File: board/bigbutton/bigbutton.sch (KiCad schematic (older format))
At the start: 55 parts, among them J1 SWD, J2 USB_C_Receptacle_USB2.0, SW1 RESET, SW2 SMOL, SW3 LORGE, U1 STM32F302CBTx, U2 ATECC608A-SSHDA, U3 WE-TVS-82400102, X1 16MHz

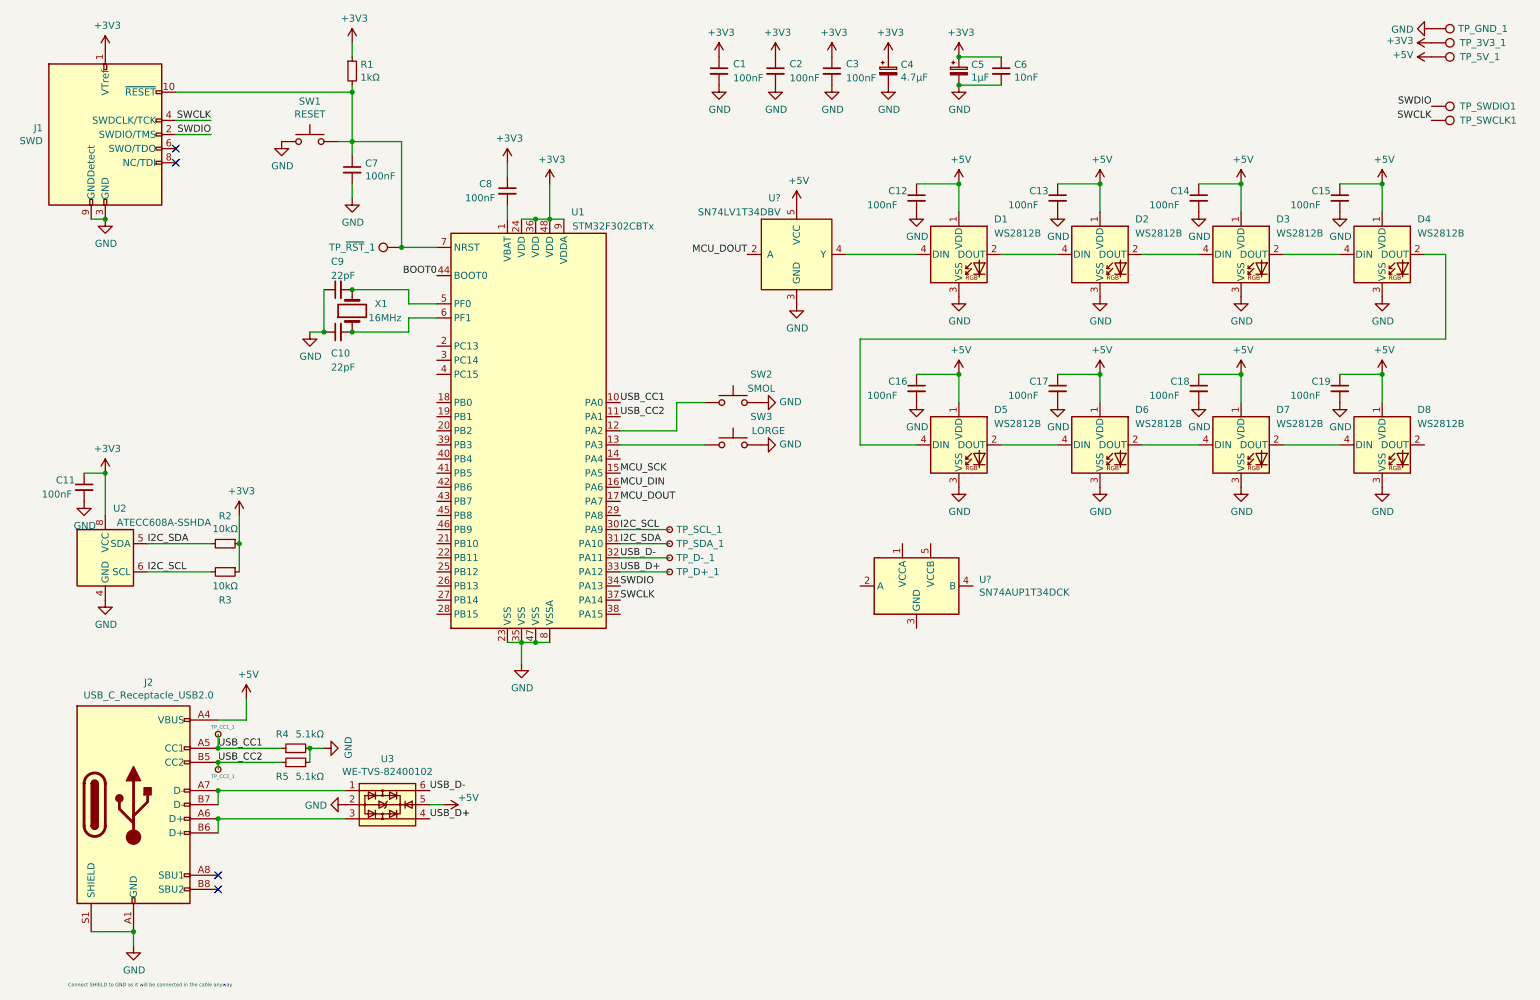
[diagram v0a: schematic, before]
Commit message: Add vreg
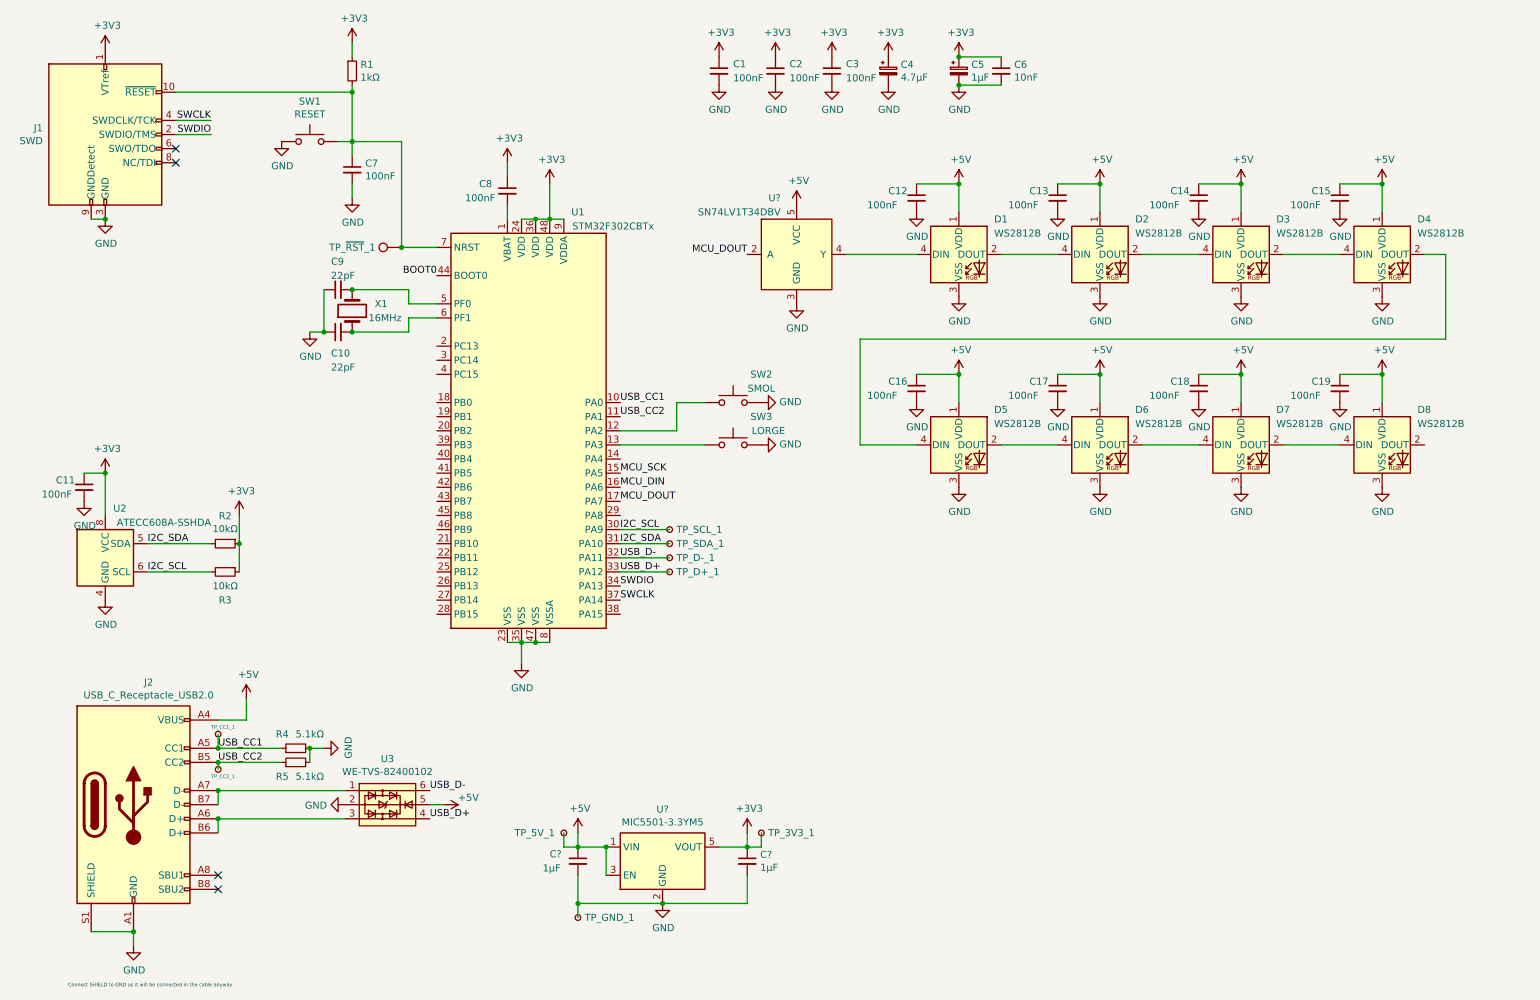
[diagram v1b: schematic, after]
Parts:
- removed TP_3V3_1, TP_5V_1, TP_GND_1, TP_SWCLK1, TP_SWDIO1: TestPoint, symbol Connector:TestPoint
- removed U?: SN74AUP1T34DCK, Package_TO_SOT_SMD:SOT-353_SC-70-5, symbol Logic_LevelTranslator:SN74AUP1T34DCK
- added C? (x2): 1µF, symbol Device:C_Small
- added TP_3V3_1, TP_5V_1, TP_GND_1: TestPoint_Small, symbol Connector:TestPoint_Small
- added U?: MIC5501-3.3YM5, Package_TO_SOT_SMD:SOT-23-5, symbol Regulator_Linear:MIC5501-3.0YM5
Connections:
- net +3V3: now also C?.1, TP_3V3_1.1, U?.5 (VOUT)
- net +5V: now also C?.1, TP_5V_1.1, U?.1 (VIN), U?.3 (EN)
- net GND: now also C?.2, C?.2, TP_GND_1.1, U?.2 (GND)
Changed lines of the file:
@@
 Text Label 4800 4150 0    50   ~ 0
 I2C_SCL
-$Comp
-L Connector:TestPoint TP_SWDIO1
-U 1 1 5F610285
-P 10550 1150
-F 0 "TP_SWDIO1" V 10550 1350 50  0000 L CNN
-F 1 "TestPoint" V 10595 1338 50  0001 L CNN
-F 2 "" H 10750 1150 50  0001 C CNN
-F 3 "~" H 10750 1150 50  0001 C CNN
-	1    10550 1150
-	0    1    1    0
-$EndComp
-$Comp
-L Connector:TestPoint TP_SWCLK1
-U 1 1 5F610307
-P 10550 1250
-F 0 "TP_SWCLK1" V 10550 1450 50  0000 L CNN
-F 1 "TestPoint" V 10595 1438 50  0001 L CNN
-F 2 "" H 10750 1250 50  0001 C CNN
-F 3 "~" H 10750 1250 50  0001 C CNN
-	1    10550 1250
-	0    1    1    0
-$EndComp
-Text Label 10550 1150 2    50   ~ 0
-SWDIO
-Text Label 10550 1250 2    50   ~ 0
-SWCLK
 Text Label 4800 4350 0    50   ~ 0
 USB_D-
@@
 Text Label 4800 3750 0    50   ~ 0
 MCU_SCK
-$Comp
-L Connector:TestPoint TP_GND_1
-U 1 1 5F63CA5F
-P 10550 600
-F 0 "TP_GND_1" V 10550 788 50  0000 L CNN
-F 1 "TestPoint" V 10595 788 50  0001 L CNN
-F 2 "" H 10750 600 50  0001 C CNN
-F 3 "~" H 10750 600 50  0001 C CNN
-	1    10550 600
-	0    1    1    0
-$EndComp
-$Comp
-L power:GND #PWR01
-U 1 1 5F63D061
-P 10550 600
-F 0 "#PWR01" H 10550 350 50  0001 C CNN
-F 1 "GND" V 10555 472 50  0000 R CNN
-F 2 "" H 10550 600 50  0001 C CNN
-F 3 "" H 10550 600 50  0001 C CNN
-	1    10550 600
-	0    1    1    0
-$EndComp
-$Comp
-L Connector:TestPoint TP_3V3_1
-U 1 1 5F63F10F
-P 10550 700
-F 0 "TP_3V3_1" V 10550 900 50  0000 L CNN
-F 1 "TestPoint" V 10595 888 50  0001 L CNN
-F 2 "" H 10750 700 50  0001 C CNN
-F 3 "~" H 10750 700 50  0001 C CNN
-	1    10550 700
-	0    1    1    0
-$EndComp
-$Comp
-L power:+3V3 #PWR03
-U 1 1 5F63F709
-P 10550 700
-F 0 "#PWR03" H 10550 550 50  0001 C CNN
-F 1 "+3V3" V 10565 828 50  0000 L CNN
-F 2 "" H 10550 700 50  0001 C CNN
-F 3 "" H 10550 700 50  0001 C CNN
-	1    10550 700
-	0    -1   -1   0
-$EndComp
-$Comp
-L Connector:TestPoint TP_5V_1
-U 1 1 5F63F82F
-P 10550 800
-F 0 "TP_5V_1" V 10550 1000 50  0000 L CNN
-F 1 "TestPoint" V 10595 988 50  0001 L CNN
-F 2 "" H 10750 800 50  0001 C CNN
-F 3 "~" H 10750 800 50  0001 C CNN
-	1    10550 800
-	0    1    1    0
-$EndComp
-$Comp
-L power:+5V #PWR09
-U 1 1 5F63FFC3
-P 10550 800
-F 0 "#PWR09" H 10550 650 50  0001 C CNN
-F 1 "+5V" V 10565 928 50  0000 L CNN
-F 2 "" H 10550 800 50  0001 C CNN
-F 3 "" H 10550 800 50  0001 C CNN
-	1    10550 800
-	0    -1   -1   0
-$EndComp
 Wire Wire Line
 	4100 1950 4200 1950
@@
 	6400 2200 6900 2200
 $Comp
-L Logic_LevelTranslator:SN74AUP1T34DCK U?
-U 1 1 5F79F9D3
-P 6900 4550
-F 0 "U?" H 7344 4596 50  0000 L CNN
-F 1 "SN74AUP1T34DCK" H 7344 4505 50  0000 L CNN
-F 2 "Package_TO_SOT_SMD:SOT-353_SC-70-5" H 6900 3850 50  0001 C CNN
-F 3 "http://www.ti.com/lit/ds/symlink/sn74aup1t34.pdf" H 6900 3950 50  0001 C CNN
-	1    6900 4550
-	1    0    0    -1
-$EndComp
-$Comp
 L bigbutton:SN74LV1T34DBV U?
 U 1 1 5F7A4DA0
@@
 	1    0    0    -1
 $EndComp
+$Comp
+L Regulator_Linear:MIC5501-3.0YM5 U?
+U 1 1 5F7ACD40
+P 5100 6500
+F 0 "U?" H 5100 6867 50  0000 C CNN
+F 1 "MIC5501-3.3YM5" H 5100 6776 50  0000 C CNN
+F 2 "Package_TO_SOT_SMD:SOT-23-5" H 5100 6100 50  0001 C CNN
+F 3 "http://ww1.microchip.com/downloads/en/DeviceDoc/MIC550X.pdf" H 4850 6750 50  0001 C CNN
+	1    5100 6500
+	1    0    0    -1
+$EndComp
+Wire Wire Line
+	4700 6400 4700 6600
+Wire Wire Line
+	4700 6400 4500 6400
+Wire Wire Line
+	4500 6400 4500 6300
+Connection ~ 4700 6400
+$Comp
+L power:+5V #PWR?
+U 1 1 5F7B4962
+P 4500 6300
+F 0 "#PWR?" H 4500 6150 50  0001 C CNN
+F 1 "+5V" H 4515 6473 50  0000 C CNN
+F 2 "" H 4500 6300 50  0001 C CNN
+F 3 "" H 4500 6300 50  0001 C CNN
+	1    4500 6300
+	1    0    0    -1
+$EndComp
+Wire Wire Line
+	5500 6400 5700 6400
+Wire Wire Line
+	5700 6400 5700 6300
+$Comp
+L power:+3V3 #PWR?
+U 1 1 5F7B7EC3
+P 5700 6300
+F 0 "#PWR?" H 5700 6150 50  0001 C CNN
+F 1 "+3V3" H 5715 6473 50  0000 C CNN
+F 2 "" H 5700 6300 50  0001 C CNN
+F 3 "" H 5700 6300 50  0001 C CNN
+	1    5700 6300
+	1    0    0    -1
+$EndComp
+$Comp
+L power:GND #PWR?
+U 1 1 5F7B8883
+P 5100 6800
+F 0 "#PWR?" H 5100 6550 50  0001 C CNN
+F 1 "GND" H 5105 6627 50  0000 C CNN
+F 2 "" H 5100 6800 50  0001 C CNN
+F 3 "" H 5100 6800 50  0001 C CNN
+	1    5100 6800
+	1    0    0    -1
+$EndComp
+$Comp
+L Device:C_Small C?
+U 1 1 5F7B9C07
+P 4500 6500
+F 0 "C?" H 4300 6550 50  0000 L CNN
+F 1 "1µF" H 4250 6450 50  0000 L CNN
+F 2 "" H 4500 6500 50  0001 C CNN
+F 3 "~" H 4500 6500 50  0001 C CNN
+	1    4500 6500
+	1    0    0    -1
+$EndComp
+Connection ~ 4500 6400
+Wire Wire Line
+	4500 6600 4500 6800
+Wire Wire Line
+	4500 6800 5100 6800
+Connection ~ 5100 6800
+Wire Wire Line
+	5100 6800 5700 6800
+Wire Wire Line
+	5700 6800 5700 6600
+$Comp
+L Device:C_Small C?
+U 1 1 5F7C0E99
+P 5700 6500
+F 0 "C?" H 5792 6546 50  0000 L CNN
+F 1 "1µF" H 5792 6455 50  0000 L CNN
+F 2 "" H 5700 6500 50  0001 C CNN
+F 3 "~" H 5700 6500 50  0001 C CNN
+	1    5700 6500
+	1    0    0    -1
+$EndComp
+Connection ~ 5700 6400
+$Comp
+L Connector:TestPoint_Small TP_5V_1
+U 1 1 5F7C43D8
+P 4400 6300
+F 0 "TP_5V_1" H 4050 6300 50  0000 L CNN
+F 1 "TestPoint_Small" H 4448 6255 50  0001 L CNN
+F 2 "" H 4600 6300 50  0001 C CNN
+F 3 "~" H 4600 6300 50  0001 C CNN
+	1    4400 6300
+	1    0    0    -1
+$EndComp
+Wire Wire Line
+	4400 6300 4400 6400
+Wire Wire Line
+	4400 6400 4500 6400
+$Comp
+L Connector:TestPoint_Small TP_GND_1
+U 1 1 5F7C7F7F
+P 4500 6900
+F 0 "TP_GND_1" H 4548 6900 50  0000 L CNN
+F 1 "TestPoint_Small" H 4548 6855 50  0001 L CNN
+F 2 "" H 4700 6900 50  0001 C CNN
+F 3 "~" H 4700 6900 50  0001 C CNN
+	1    4500 6900
+	1    0    0    -1
+$EndComp
+Wire Wire Line
+	4500 6800 4500 6900
+Connection ~ 4500 6800
+$Comp
+L Connector:TestPoint_Small TP_3V3_1
+U 1 1 5F7CBAA6
+P 5800 6300
+F 0 "TP_3V3_1" H 5848 6300 50  0000 L CNN
+F 1 "TestPoint_Small" H 5848 6255 50  0001 L CNN
+F 2 "" H 6000 6300 50  0001 C CNN
+F 3 "~" H 6000 6300 50  0001 C CNN
+	1    5800 6300
+	1    0    0    -1
+$EndComp
+Wire Wire Line
+	5800 6300 5800 6400
+Wire Wire Line
+	5800 6400 5700 6400
 $EndSCHEMATC
